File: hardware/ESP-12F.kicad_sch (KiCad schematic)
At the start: 26 parts, among them U5 ESP-12F, U7 PI4IOE5V6416LEX, U8 PI4IOE5V6416LEX, U9 MCP2558FD-xMF

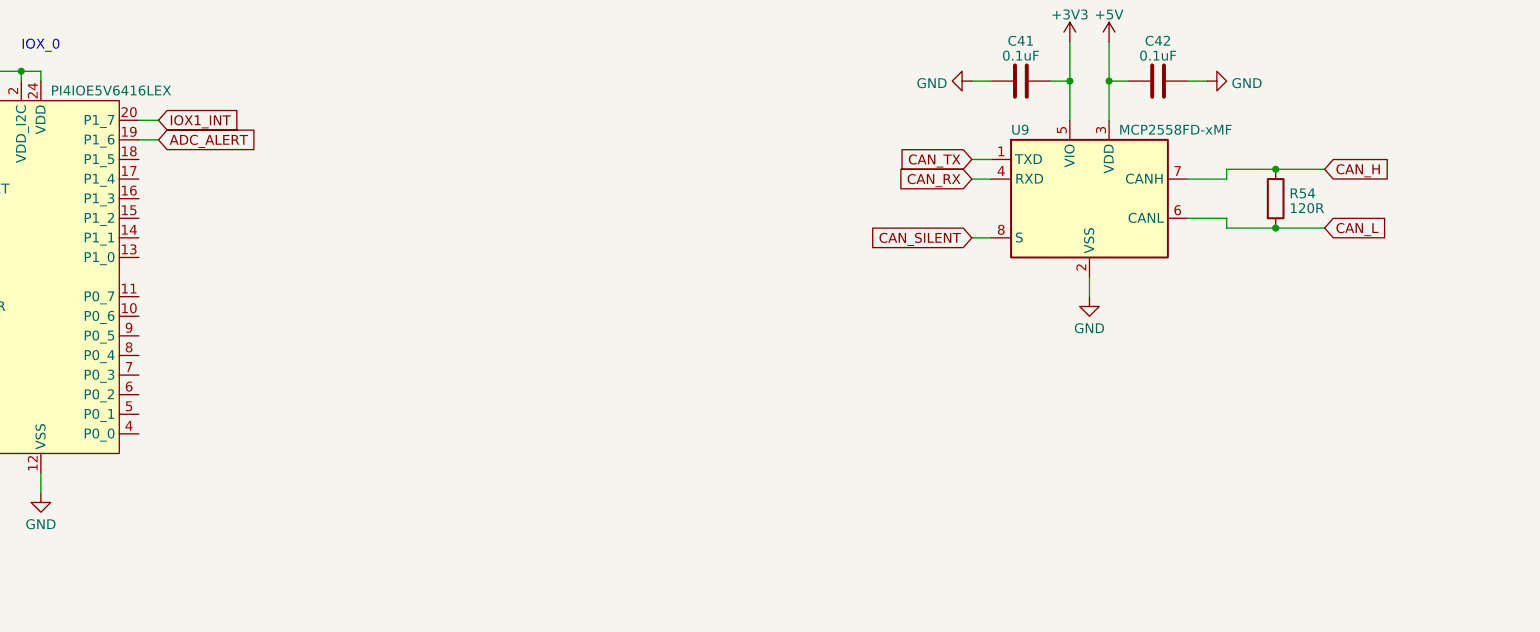
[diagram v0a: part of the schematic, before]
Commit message: finnished rudimentry schimatics still needs alot of work
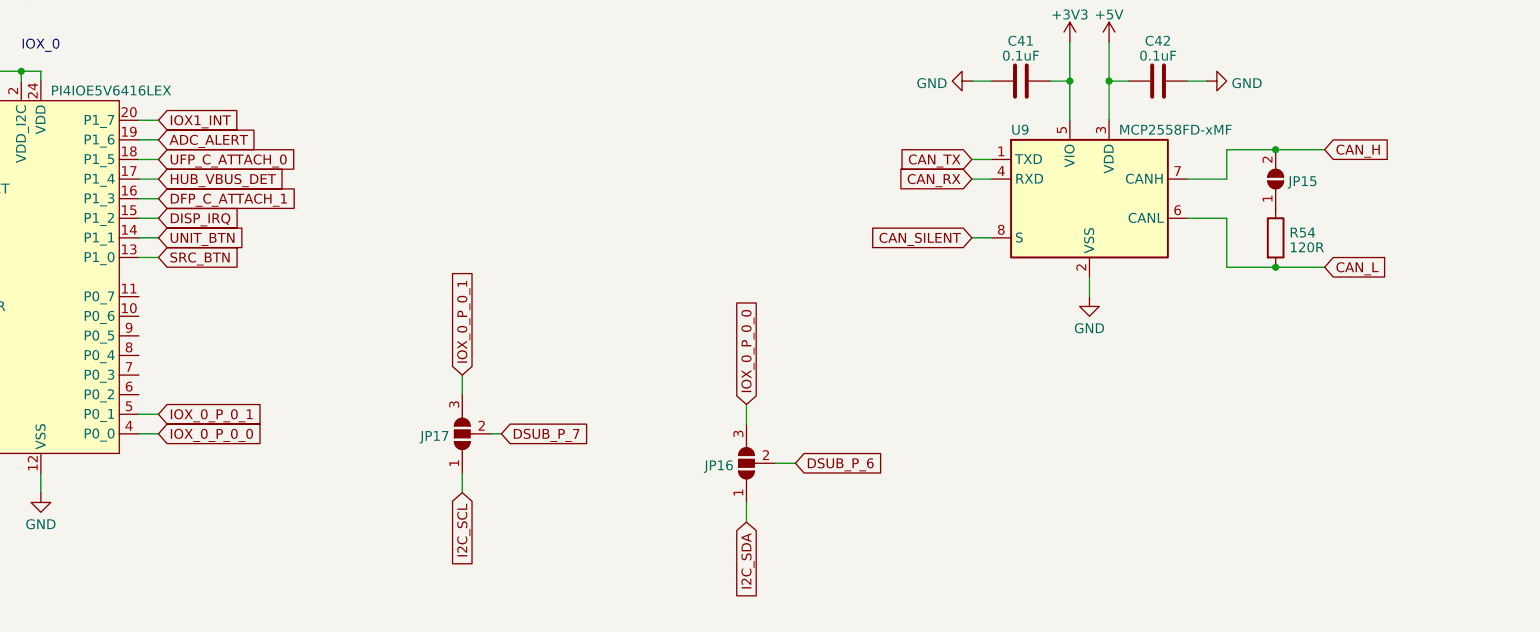
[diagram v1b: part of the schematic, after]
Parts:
- added JP15: ~, symbol Jumper:SolderJumper_2_Open
- added JP16, JP17: ~, symbol Jumper:SolderJumper_3_Open
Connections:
- net CAN_H: now also JP15.2 (B); no longer R54.1
- net I2C_SCL: now also JP17.1 (A)
- net I2C_SDA: now also JP16.1 (A)
- net SRC_BTN: now reaches U7.13 (P1_0)
- net UNIT_BTN: now reaches U7.14 (P1_1)
- net DISP_IRQ: now reaches U7.15 (P1_2)
- net DFP_C_ATTACH_1: now reaches U7.16 (P1_3)
- net HUB_VBUS_DET: now reaches U7.17 (P1_4)
- net UFP_C_ATTACH_0: now reaches U7.18 (P1_5)
- net IOX_0_P_0_0: now reaches U7.4 (P0_0)
- net IOX_0_P_0_0: now also JP16.3 (B)
- net IOX_0_P_0_1: now reaches U7.5 (P0_1)
- net IOX_0_P_0_1: now also JP17.3 (B)
- new net: JP15.1 (A), R54.1
- new net DSUB_P_6: JP16.2 (C)
- new net DSUB_P_7: JP17.2 (C)
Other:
- moved on the sheet: R54
